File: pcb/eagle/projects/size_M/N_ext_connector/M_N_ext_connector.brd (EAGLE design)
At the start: 10 parts, among them J1 RJ11

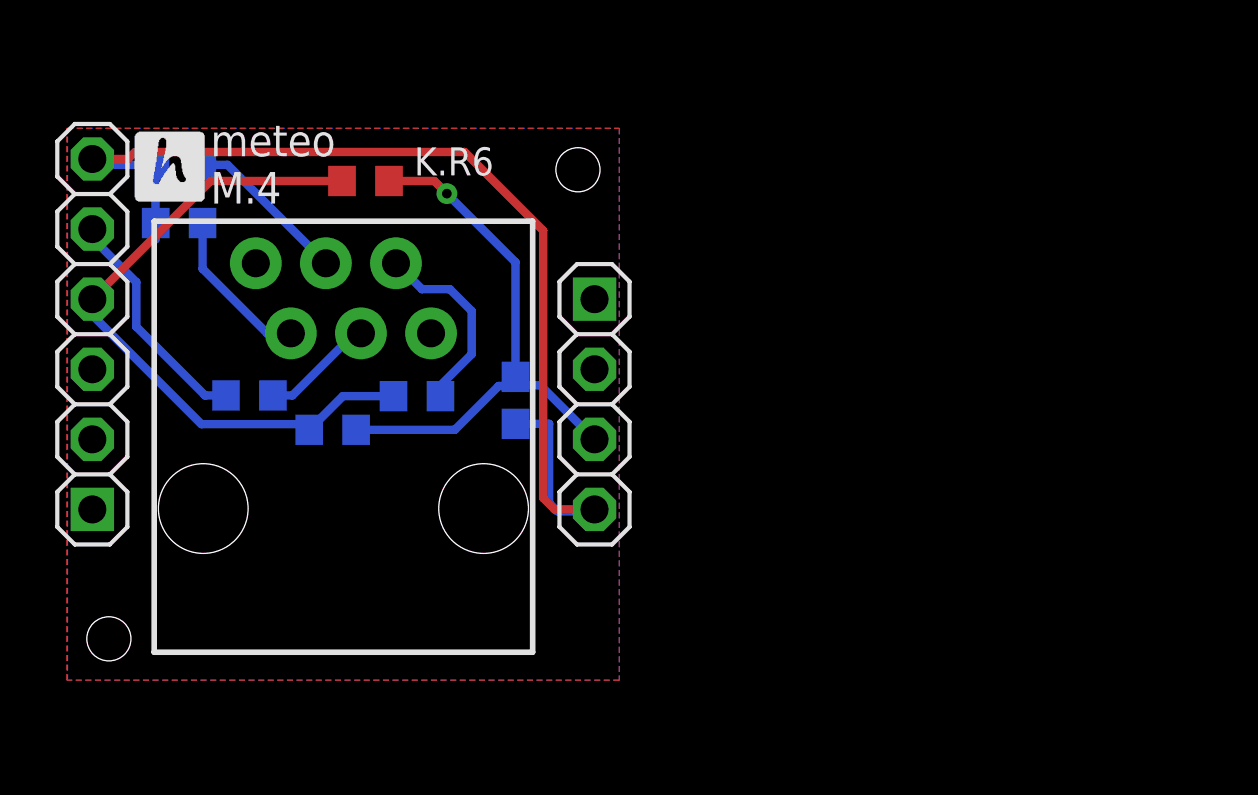
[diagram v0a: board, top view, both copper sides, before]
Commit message: PCB v4
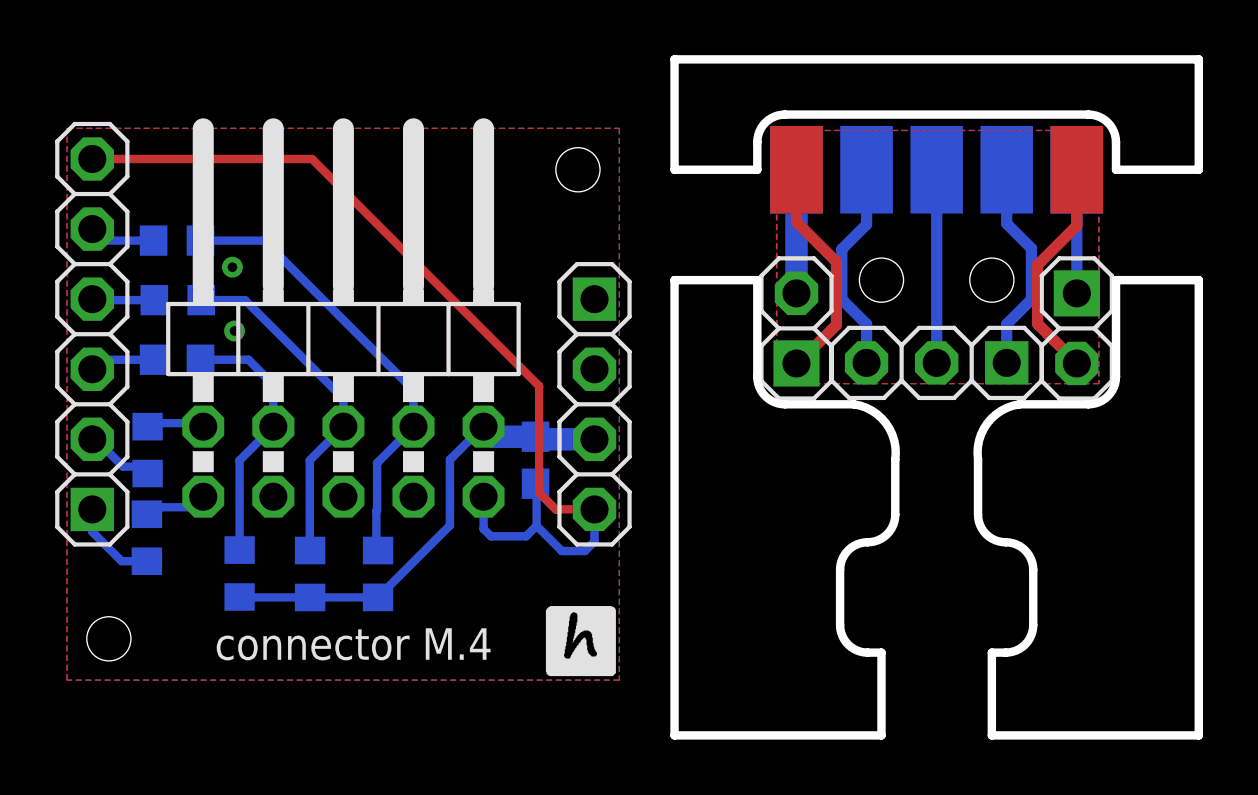
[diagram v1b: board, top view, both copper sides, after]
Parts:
- removed J1: RJ11, SparkFun-Connectors:RJ11-6
- removed K.C1: 100n, rcl:C0603
- removed K.R1, K.R3, K.R4, K.R5: 1k, rcl:R0603
- removed K.R2, K.R6: 4k7, rcl:R0603
- added JP1: (no value), pinhead2:1X03
- added JP4: (no value), pinhead2:2X05/90
- added JP5, JP6: (no value), pinhead2:1X02
- added N.C1: 100n, rcl:C0603
- added N.R1, N.R2, N.R3, N.R4, N.R5, N.R6, N.R7, N.R8: 4k7, rcl:R0603
- added U$1: 7PIN_CONNECTOR, hugo:7PIN_CONNECTOR
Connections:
- new net GND1: JP5.1, U$1.7
- new net N$10: JP4.2, N.R7.2
- new net N$11: JP4.1, N.R8.2
- new net N$12: JP1.2, U$1.4
- new net N$13: JP1.3, U$1.5
- new net N$14: JP6.1, U$1.2
- new net N$15: JP6.2, U$1.1
- new net N$4: JP2.5, N.R4.1
- new net N$5: JP2.4, N.R5.1
- new net N$9: JP4.4, N.R3.2, N.R6.2
- new net VCC1: JP5.2, U$1.6
- net GND: now also JP4.9, N.C1.2; no longer K.C1.2, K.R1.1, K.R5.1
- net N$1: now also JP1.1, U$1.3; no longer J1.5, K.R4.2
- net N$2: now also JP4.8, N.R1.2, N.R4.2; no longer JP2.5, K.R3.1
- net N$3: now also JP4.6, N.R2.2, N.R5.2; no longer JP2.4, K.R2.2, K.R4.1, K.R6.2
- net N$6: now also JP2.3, N.R6.1; no longer J1.4, K.R3.2
- net N$7: now also JP2.2, N.R7.1; no longer J1.3, K.R5.2
- net N$8: now also JP2.1, N.R8.1; no longer J1.2, K.R1.2
- net VCC: now also JP4.10, N.C1.1, N.R1.1, N.R2.1, N.R3.1; no longer K.C1.1, K.R2.1, K.R6.1
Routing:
- net N$3: track 24.5 -> 12.8 mm
- net N$9: track 0.00 -> 9.73 mm
- net N$13: track 0.00 -> 8.39 mm
- net GND1: track 0.00 -> 8.25 mm
- net N$15: track 0.00 -> 8.20 mm
- net N$2: track 8.48 -> 16.4 mm
- net N$12: track 0.00 -> 7.00 mm
- net GND: track 40.3 -> 34.5 mm, vias 0 -> 2
- net VCC1: track 0.00 -> 4.48 mm
- net N$14: track 0.00 -> 4.48 mm
- net N$7: track 5.95 -> 2.52 mm
- net VCC: track 20.3 -> 17.0 mm, vias 1 -> 0
- net N$8: track 5.82 -> 3.23 mm
- net N$4: track 0.00 -> 2.39 mm
- net N$11: track 0.00 -> 2.31 mm
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- added copper zone on layer 1, net GND1
- added copper zone on layer 16, net GND1
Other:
- board outline added: 19 x 24.5 mm
- board text added: "connector M.4"
- board text removed: "meteo M.4"
